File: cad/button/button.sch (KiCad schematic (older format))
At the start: 17 parts, among them J1 uSD_SPI, J2 SWD, SW1 SW_Push, U1 STM32L072KZTx, U2 PAM8302AAS

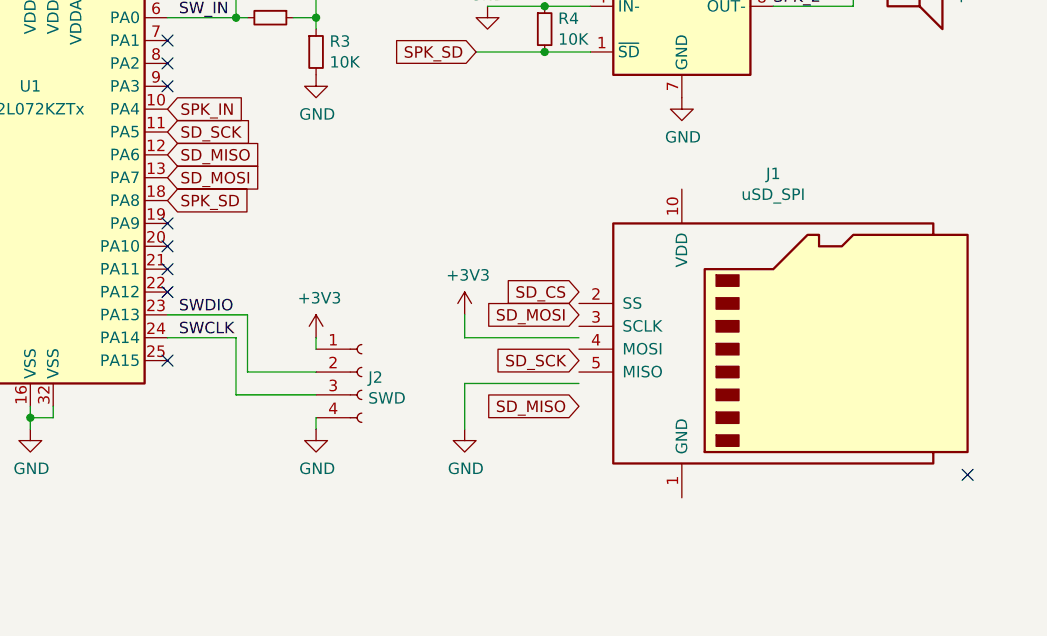
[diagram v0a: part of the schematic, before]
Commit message: more drawing
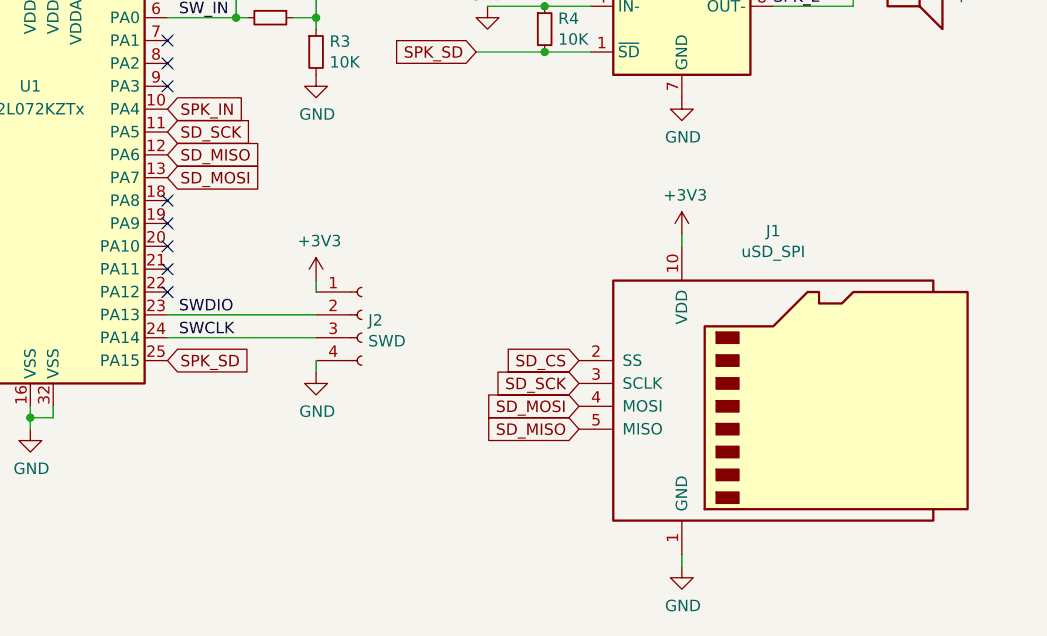
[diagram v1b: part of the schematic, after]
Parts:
- J1: footprint Connectors:microSD_Card_Receptacle_Wuerth_693072010801 -> custom:PJRC_uSD_Adapter
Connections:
- wire segments 59 -> 53
- no-connect marks 17 -> 16
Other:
- moved on the sheet: J1, J2
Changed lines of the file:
@@
 NoConn ~ 3250 3600
 NoConn ~ 3250 3700
-NoConn ~ 3250 4000
 NoConn ~ 2150 3100
 NoConn ~ 2150 3200
@@
 L Connector:Conn_01x04_Female J2
 U 1 1 5C3A9A62
-P 4100 4050
-F 0 "J2" H 4128 4026 50  0000 L CNN
-F 1 "SWD" H 4128 3935 50  0000 L CNN
-F 2 "custom:Pad_4contacts" H 4100 4050 50  0001 C CNN
-F 3 "~" H 4100 4050 50  0001 C CNN
-	1    4100 4050
+P 4100 3800
+F 0 "J2" H 4128 3776 50  0000 L CNN
+F 1 "SWD" H 4128 3685 50  0000 L CNN
+F 2 "custom:Pad_4contacts" H 4100 3800 50  0001 C CNN
+F 3 "~" H 4100 3800 50  0001 C CNN
+	1    4100 3800
 	1    0    0    -1
 $EndComp
@@
 L power:GND #PWR0101
 U 1 1 5C3AA417
-P 3900 4300
-F 0 "#PWR0101" H 3900 4050 50  0001 C CNN
-F 1 "GND" H 3905 4127 50  0000 C CNN
-F 2 "" H 3900 4300 50  0001 C CNN
-F 3 "" H 3900 4300 50  0001 C CNN
-	1    3900 4300
+P 3900 4050
+F 0 "#PWR0101" H 3900 3800 50  0001 C CNN
+F 1 "GND" H 3905 3877 50  0000 C CNN
+F 2 "" H 3900 4050 50  0001 C CNN
+F 3 "" H 3900 4050 50  0001 C CNN
+	1    3900 4050
 	1    0    0    -1
 $EndComp
@@
 L power:+3V3 #PWR0106
 U 1 1 5C3AA5DA
-P 3900 3900
-F 0 "#PWR0106" H 3900 3750 50  0001 C CNN
-F 1 "+3V3" H 3915 4073 50  0000 C CNN
-F 2 "" H 3900 3900 50  0001 C CNN
-F 3 "" H 3900 3900 50  0001 C CNN
-	1    3900 3900
+P 3900 3650
+F 0 "#PWR0106" H 3900 3500 50  0001 C CNN
+F 1 "+3V3" H 3915 3823 50  0000 C CNN
+F 2 "" H 3900 3650 50  0001 C CNN
+F 3 "" H 3900 3650 50  0001 C CNN
+	1    3900 3650
 	1    0    0    -1
 $EndComp
@@
 Text Label 1850 2700 0    50   ~ 0
 BOOT0
-Wire Wire Line
-	3250 3800 3600 3800
-Wire Wire Line
-	3250 3900 3550 3900
 $Comp
 L custom:uSD_SPI J1
 U 1 1 5C3DB7D2
-P 5950 3900
-F 0 "J1" H 5900 4617 50  0000 C CNN
-F 1 "uSD_SPI" H 5900 4526 50  0000 C CNN
-F 2 "Connectors:microSD_Card_Receptacle_Wuerth_693072010801" H 7100 4200 50  0001 C CNN
-F 3 "http://katalog.we-online.de/em/datasheet/693072010801.pdf" H 5950 3900 50  0001 C CNN
-	1    5950 3900
+P 5950 4150
+F 0 "J1" H 5900 4867 50  0000 C CNN
+F 1 "uSD_SPI" H 5900 4776 50  0000 C CNN
+F 2 "custom:PJRC_uSD_Adapter" H 7100 4450 50  0001 C CNN
+F 3 "http://katalog.we-online.de/em/datasheet/693072010801.pdf" H 5950 4150 50  0001 C CNN
+	1    5950 4150
 	1    0    0    -1
 $EndComp
@@
 Text GLabel 3250 2900 2    50   Input ~ 0
 SPK_IN
-Text GLabel 3250 3300 2    50   Input ~ 0
+Text GLabel 3250 4000 2    50   Input ~ 0
 SPK_SD
 Text GLabel 5100 2250 0    50   Input ~ 0
 SPK_IN
-Text GLabel 5050 3700 0    50   Input ~ 0
+Text GLabel 5050 4000 0    50   Input ~ 0
 SD_CS
-Text GLabel 5050 4000 0    50   Input ~ 0
+Text GLabel 5050 4100 0    50   Input ~ 0
 SD_SCK
+Text GLabel 5050 4300 0    50   Input ~ 0
+SD_MISO
 Text GLabel 5050 4200 0    50   Input ~ 0
-SD_MISO
-Text GLabel 5050 3800 0    50   Input ~ 0
 SD_MOSI
-Wire Wire Line
-	5050 3900 4550 3900
-Wire Wire Line
-	4550 3900 4550 3800
-Wire Wire Line
-	5050 4100 4550 4100
 $Comp
 L power:GND #PWR0115
 U 1 1 5C3DDAEF
-P 4550 4300
-F 0 "#PWR0115" H 4550 4050 50  0001 C CNN
-F 1 "GND" H 4555 4127 50  0000 C CNN
-F 2 "" H 4550 4300 50  0001 C CNN
-F 3 "" H 4550 4300 50  0001 C CNN
-	1    4550 4300
+P 5500 4900
+F 0 "#PWR0115" H 5500 4650 50  0001 C CNN
+F 1 "GND" H 5505 4727 50  0000 C CNN
+F 2 "" H 5500 4900 50  0001 C CNN
+F 3 "" H 5500 4900 50  0001 C CNN
+	1    5500 4900
 	1    0    0    -1
 $EndComp
@@
 L power:+3V3 #PWR0116
 U 1 1 5C3DDB14
-P 4550 3800
-F 0 "#PWR0116" H 4550 3650 50  0001 C CNN
-F 1 "+3V3" H 4565 3973 50  0000 C CNN
-F 2 "" H 4550 3800 50  0001 C CNN
-F 3 "" H 4550 3800 50  0001 C CNN
-	1    4550 3800
-	1    0    0    -1
-$EndComp
-NoConn ~ 6750 4500
+P 5500 3450
+F 0 "#PWR0116" H 5500 3300 50  0001 C CNN
+F 1 "+3V3" H 5515 3623 50  0000 C CNN
+F 2 "" H 5500 3450 50  0001 C CNN
+F 3 "" H 5500 3450 50  0001 C CNN
+	1    5500 3450
+	1    0    0    -1
+$EndComp
 Wire Wire Line
 	1450 2700 1450 2750
@@
 	2650 4250 2650 4300
 Wire Wire Line
-	3900 3900 3900 3950
-Wire Wire Line
-	3900 4250 3900 4300
-Wire Wire Line
-	3900 4150 3550 4150
-Wire Wire Line
-	3550 3900 3550 4150
-Wire Wire Line
-	3900 4050 3600 4050
-Wire Wire Line
-	3600 3800 3600 4050
-Wire Wire Line
-	4550 4100 4550 4300
+	3900 3650 3900 3700
+Wire Wire Line
+	3900 4000 3900 4050
+Wire Wire Line
+	5500 3450 5500 3500
+Wire Wire Line
+	5500 4850 5500 4900
+NoConn ~ 3250 3300
+Wire Wire Line
+	3250 3900 3900 3900
+Wire Wire Line
+	3250 3800 3900 3800
 $EndSCHEMATC

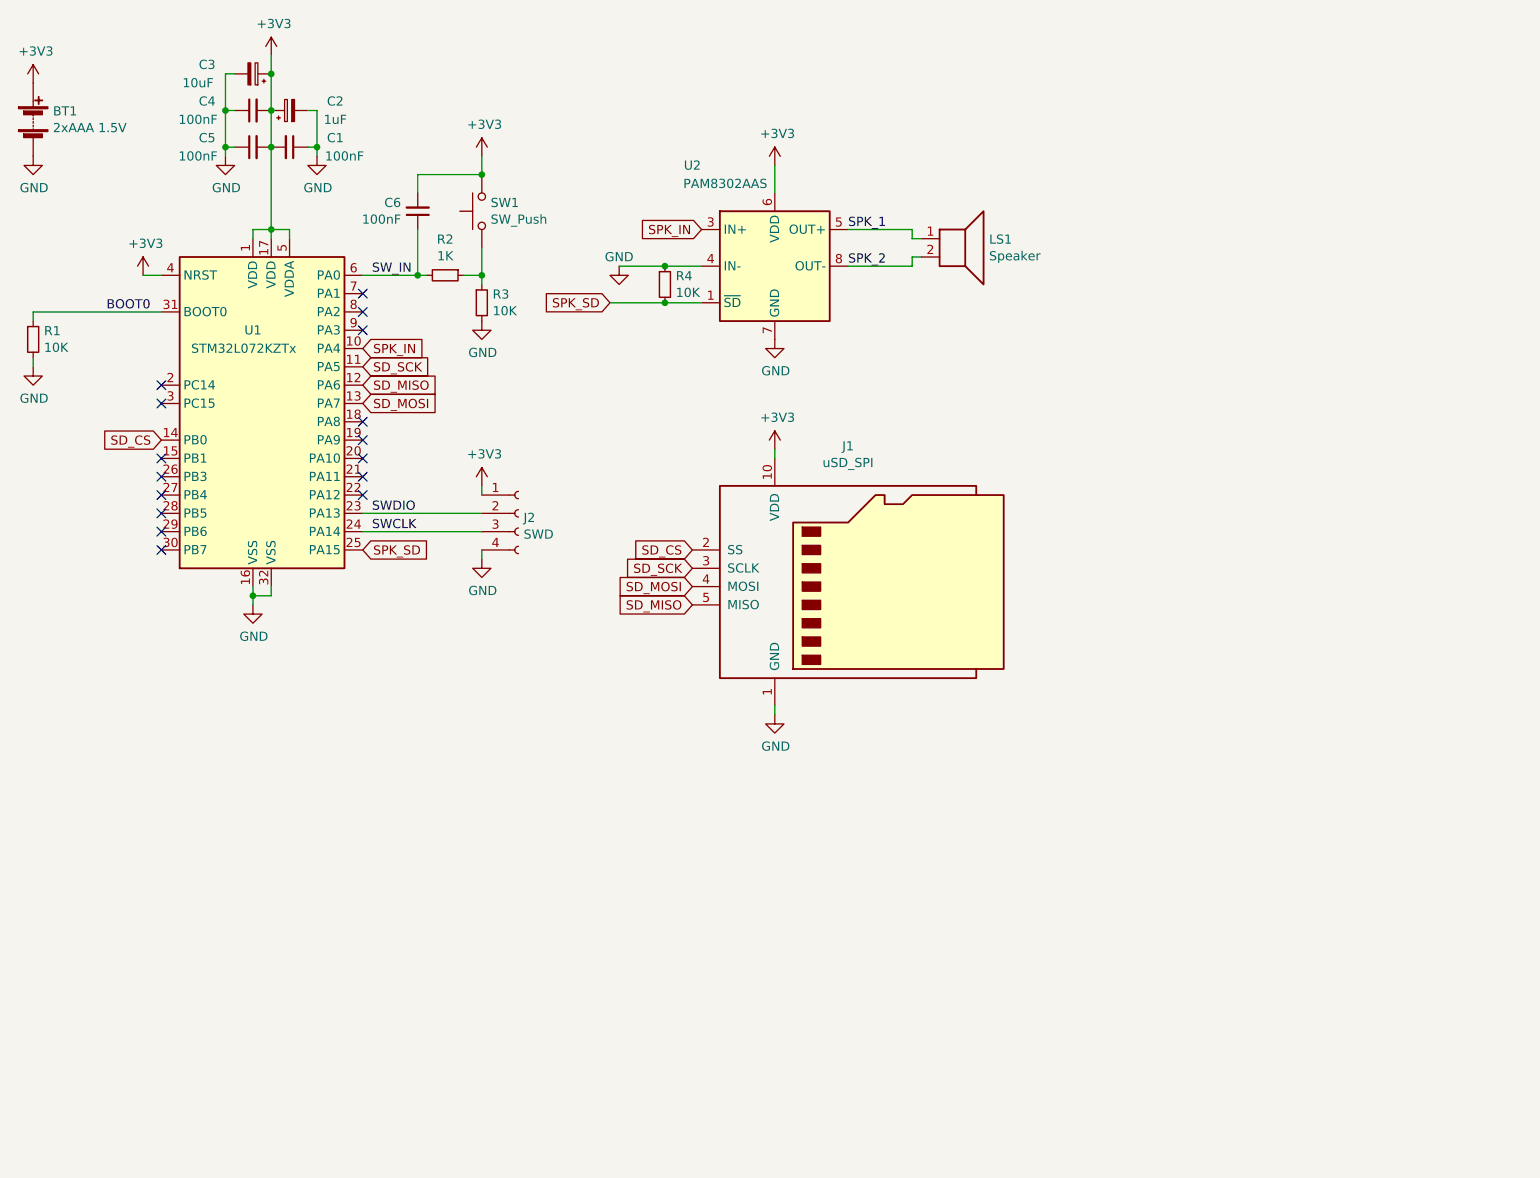
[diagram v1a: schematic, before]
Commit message: finish up schematic
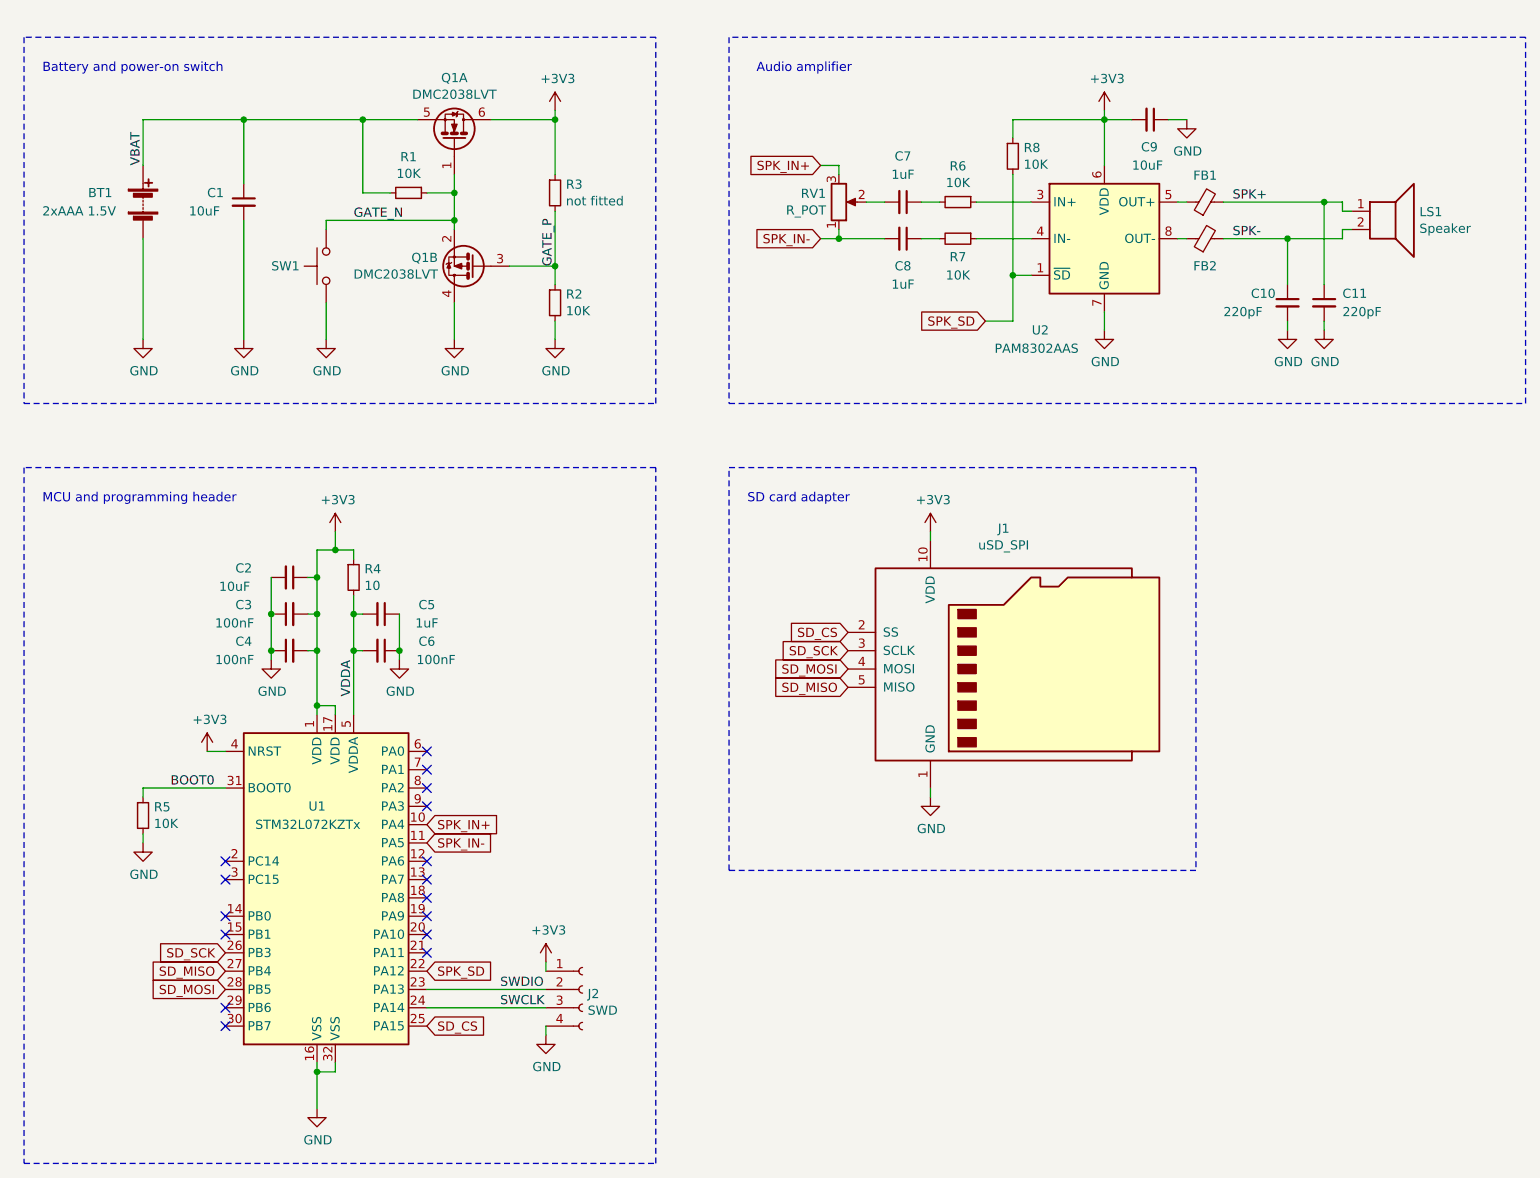
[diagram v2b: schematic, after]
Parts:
- removed C2: 1uF, Capacitors_SMD:C_0603_HandSoldering, symbol Device:CP_Small
- removed C3: 10uF, Capacitors_SMD:C_0603_HandSoldering, symbol Device:CP_Small
- removed C6: 100nF, Capacitors_SMD:C_0603_HandSoldering, symbol Device:C_Small
- added C1, C2, C9: 10uF, Capacitors_SMD:C_0603_HandSoldering, symbol Device:C_Small
- added C10, C11: 220pF, Capacitors_SMD:C_0603_HandSoldering, symbol Device:C_Small
- added C5, C7, C8: 1uF, Capacitors_SMD:C_0603_HandSoldering, symbol Device:C_Small
- added FB1, FB2: Ferrite_Bead_Small, Resistors_SMD:R_0603_HandSoldering, symbol Device:Ferrite_Bead_Small
- added Q1: DMC2038LVT, TO_SOT_Packages_SMD:TSOT-23-6, symbol custom:DMC2038LVT
- added R1, R6, R7: 10K, Resistors_SMD:R_0603_HandSoldering, symbol Device:R_Small
- added R4: 10, Resistors_SMD:R_0603_HandSoldering, symbol Device:R_Small
- added RV1: R_POT, Potentiometers:Potentiometer_Trimmer-EVM3E, symbol Device:R_POT
- R2: value 1K -> 10K
- R3: value 10K -> not fitted
- SW1: value SW_Push -> Button
- renumbered C4 to C3, C5 to C4, C1 to C6, R1 to R5, R4 to R8
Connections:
- net +3V3: now also R3.1, R8.1, C2.1, C9.2, Q1.6 (D), R4.1; no longer BT1.1 (+), C6.2, SW1.2, U1.5 (VDDA)
- net GND: now also R2.2, SW1.2, C1.2, C10.2, C11.2, C2.2, C5.1, C9.1, Q1.4 (D); no longer R3.2, R8.1, U2.4 (IN-)
- net SD_CS: now also U1.25 (PA15); no longer U1.14 (PB0)
- net SD_MISO: now also U1.27 (PB4); no longer U1.12 (PA6)
- net SD_MOSI: now also U1.28 (PB5); no longer U1.13 (PA7)
- net SD_SCK: now also U1.26 (PB3); no longer U1.11 (PA5)
- net SPK_SD: now also U1.22 (PA12); no longer U1.25 (PA15)
- net SPK_1: no longer names the net of U2.5 (OUT+)
- net SPK_1: now also FB1.1; no longer LS1.1
- net SPK_2: no longer names the net of U2.8 (OUT-)
- net SPK_2: now also FB2.1; no longer LS1.2
- net SPK_IN: no longer names the net of U2.3 (IN+)
- net SPK_IN: now also R6.1; no longer U1.10 (PA4)
- net SW_IN: no longer names the net of U1.6 (PA0)
- net SW_IN: no longer R2.2
- new net: R7.1, U2.4 (IN-)
- new net: C7.2, RV1.2
- new net: C7.1, R6.2
- new net: C8.1, R7.2
- new net GATE_N: Q1.1 (G), Q1.2 (S), R1.1, SW1.1
- new net GATE_P: Q1.3 (G), R2.1, R3.2
- new net SPK+: C11.1, FB1.2, LS1.1
- new net SPK-: C10.1, FB2.2, LS1.2
- new net SPK_IN+: RV1.3, U1.10 (PA4)
- new net SPK_IN-: C8.2, RV1.1, U1.11 (PA5)
- new net VBAT: BT1.1 (+), C1.1, Q1.5 (S), R1.2
- new net VDDA: C5.2, C6.2, R4.2, U1.5 (VDDA)
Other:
- note added: "Audio amplifier"
- note added: "Battery and power-on switch"
- note added: "MCU and programming header"
- note added: "SD card adapter"
- moved on the sheet: BT1, C3, C4, C6, J1, J2, LS1, R5, R8, SW1, U1, U2
